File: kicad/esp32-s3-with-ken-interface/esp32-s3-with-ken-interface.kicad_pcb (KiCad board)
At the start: 4 copper layers, 50.8 x 81.3 mm, 40 parts, among them J1 TYPE-C-31-M-12, Q1 UMH3N, SW1 TSC015A03526A, SW2 TSC015A03526A, SW3 TSC015A03526A, U1 CH340C, U2 AMS1117-3.3, U3 XDZ254-2-15-W-2.5-G1, U4 ESP32-S3-WROOM-1, U5 PM254-2-15-W-8.5

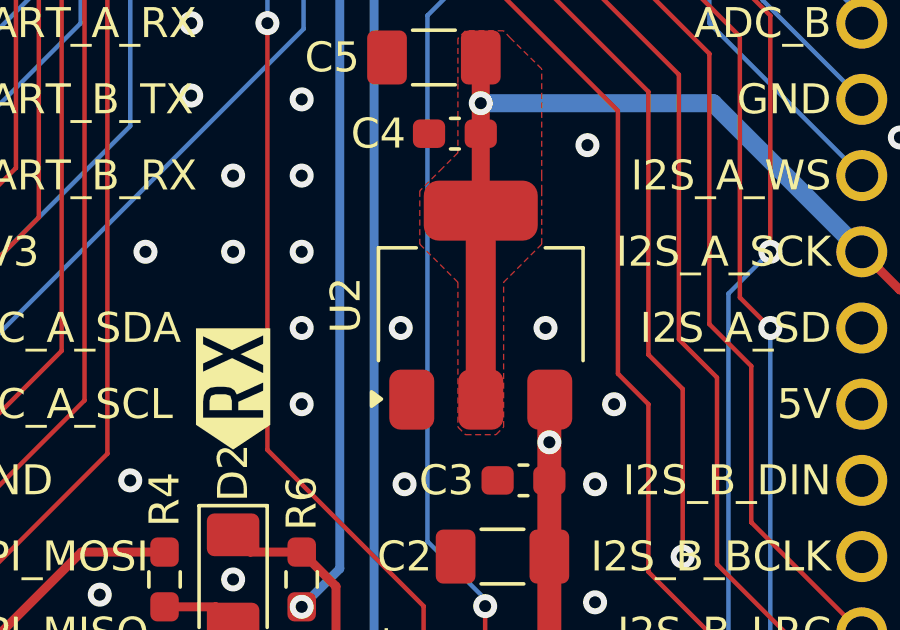
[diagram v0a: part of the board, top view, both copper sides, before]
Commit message: update symbol
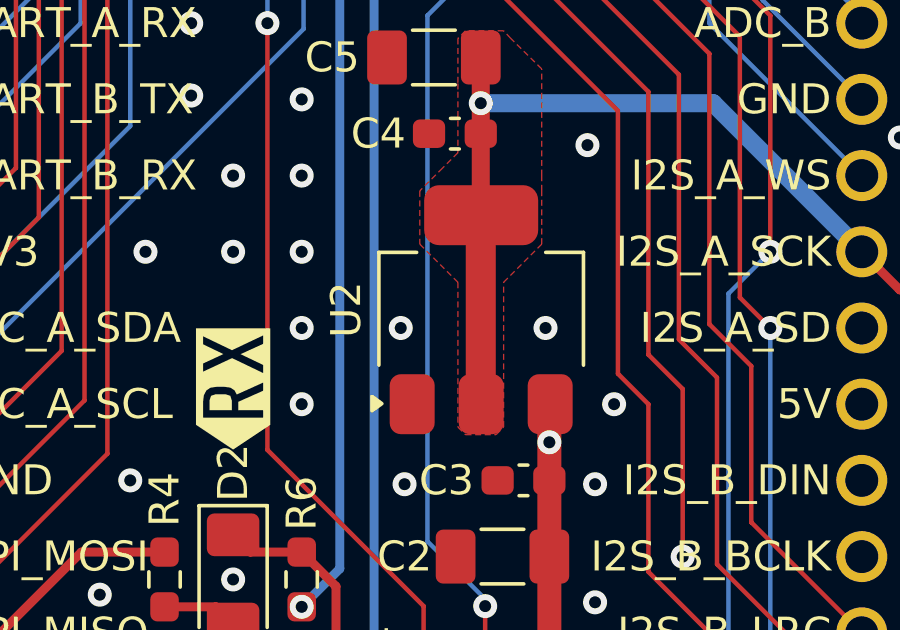
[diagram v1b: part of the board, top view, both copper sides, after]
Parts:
- moved U2 0.15 mm to (83.8, 83.5)
